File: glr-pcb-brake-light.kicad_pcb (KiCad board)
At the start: 2 copper layers, 156 x 26 mm, 31 parts, among them J1 Conn_01x04_Pin

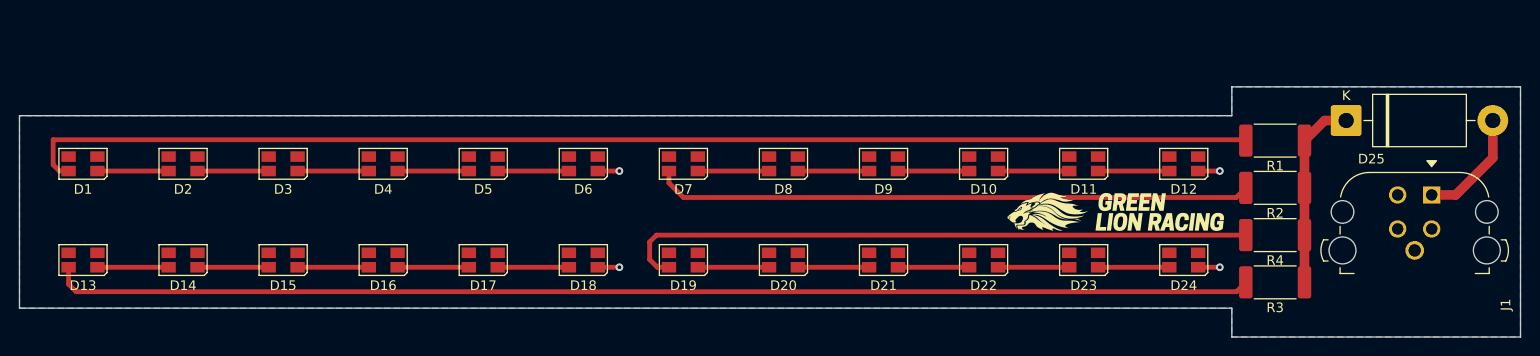
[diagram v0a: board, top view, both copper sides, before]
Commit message: pcb umdesigned fast fertig
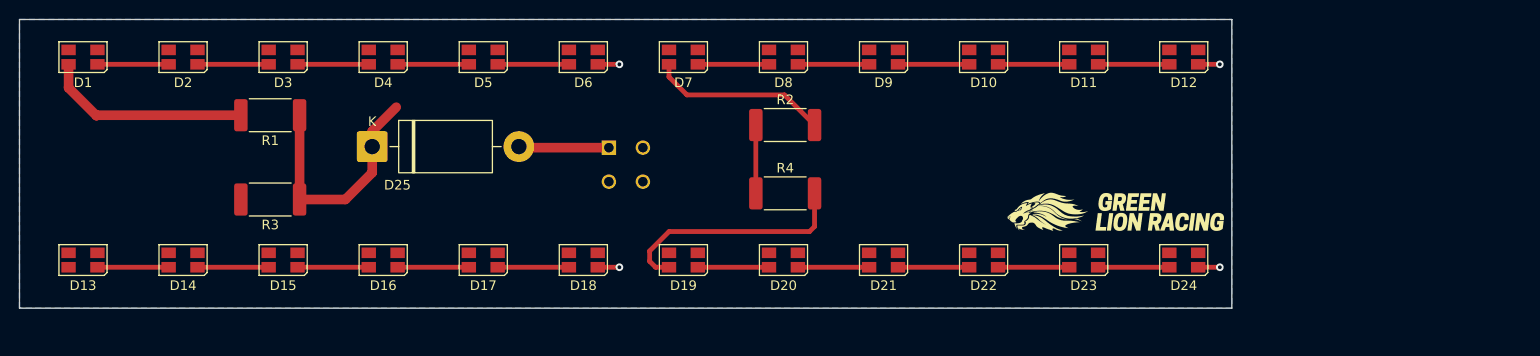
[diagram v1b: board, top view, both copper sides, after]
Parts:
- J1: footprint GLR_KiCad_Library:Wuerth_M12-Right-Angled-THT -> GLR_KiCad_Library:Wuerth_M12-Panel-Cut-THT; moved to B.Cu
- moved R3 104.8 mm to (126.1, 98.3)
- moved R1 104.5 mm to (126.1, 89.6)
- moved D25 101.3 mm to (136.7, 92.8)
- moved J1 85.7 mm to (161.3, 93.0), turned to 180 degrees
- moved R2 51.3 mm to (179.6, 90.6), turned to 0 degrees
- moved R4 51.1 mm to (179.6, 97.7), turned to 0 degrees
- moved D1 11.1 mm to (106.6, 83.5)
- moved D10 11.1 mm to (200.2, 83.5)
- moved D11 11.1 mm to (210.6, 83.5)
- moved D12 11.1 mm to (221.0, 83.5)
- moved D2 11.1 mm to (117.0, 83.5)
- moved D3 11.1 mm to (127.4, 83.5)
- moved D4 11.1 mm to (137.8, 83.5)
- moved D5 11.1 mm to (148.2, 83.5)
- moved D6 11.1 mm to (158.6, 83.5)
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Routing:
- net Net-(D13-A): track 124.8 -> 0.00 mm
- net Net-(D1-A): track 128.3 -> 21.6 mm
- net Net-(D7-A): track 62.2 -> 18.5 mm
- net Net-(D19-A): track 66.4 -> 25.0 mm
- net Net-(D25-K): track 19.9 -> 32.4 mm
- net +24V: track 11.8 -> 9.40 mm
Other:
- board size 156 x 26 mm -> 126 x 30 mm
